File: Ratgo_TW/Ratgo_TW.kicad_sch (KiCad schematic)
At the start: 11 parts, among them J1 10118193-0001LF, J2 Screw_Terminal_01x03, J3 Conn_01x04, Q1 2N7002, Q2 AO3400A, SW1 SW_Push, SW2 SW_Push, U3 AP2112K-3.3, U4 ESP-12F

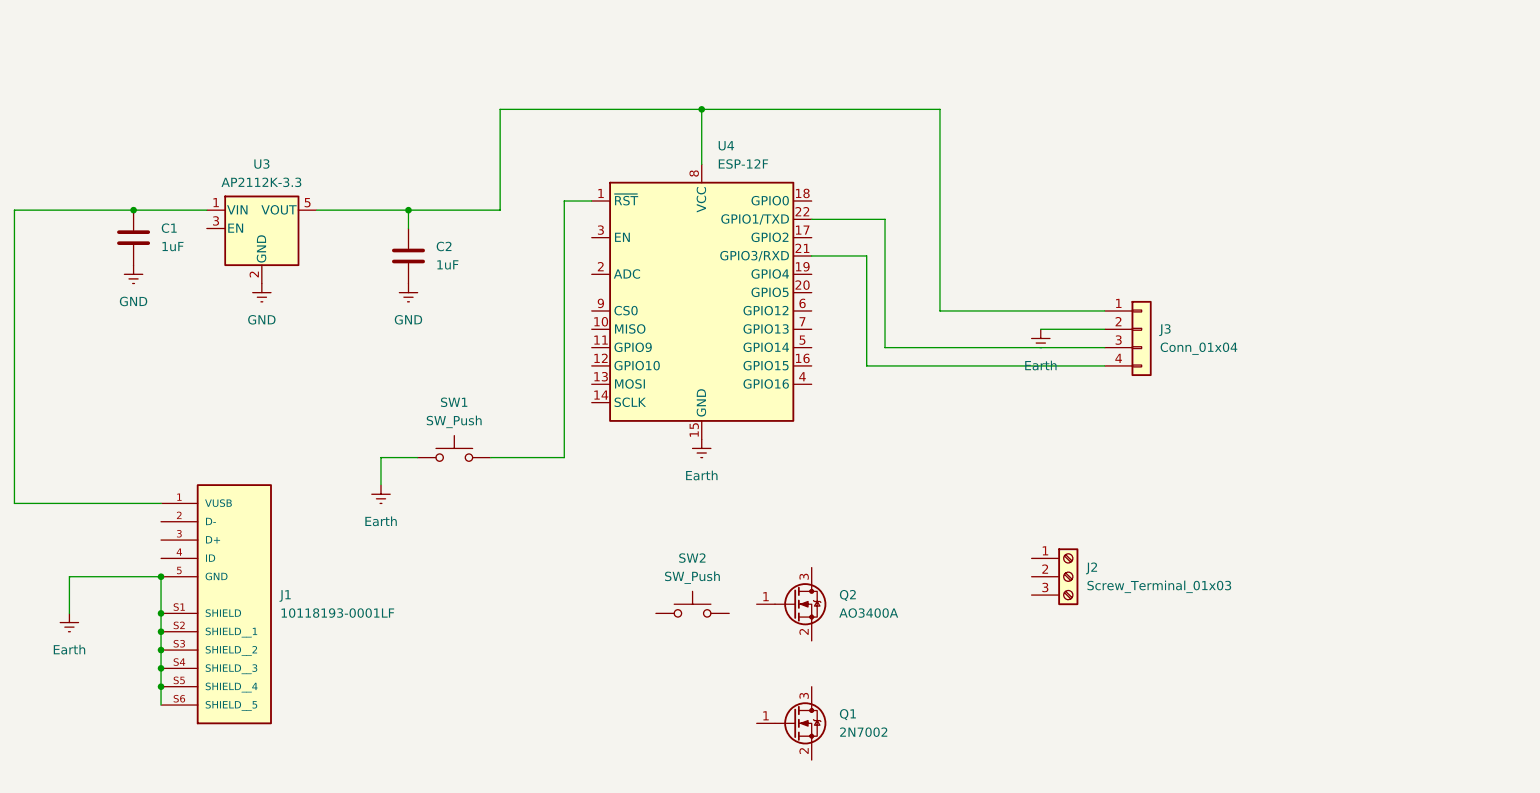
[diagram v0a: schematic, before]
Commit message: latest with all footprints
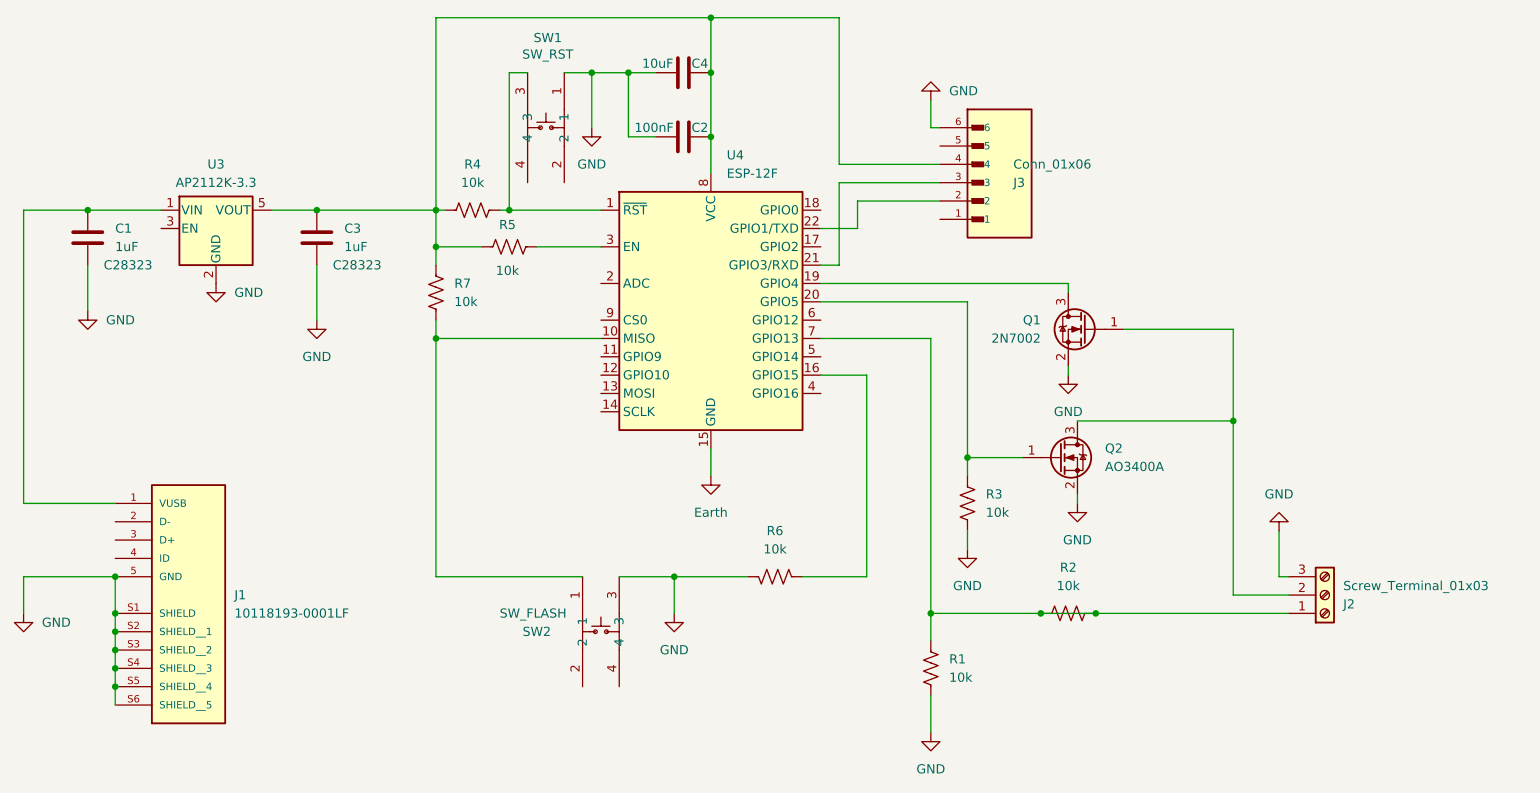
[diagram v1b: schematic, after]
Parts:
- added C3: 1uF, Capacitor_SMD:C_0805_2012Metric, symbol Device:C
- added C4: 10uF, Capacitor_SMD:C_0805_2012Metric, symbol Device:C
- added R1, R2, R3, R4, R5, R6, R7: 10k, Resistor_SMD:R_0805_2012Metric, symbol Device:R_US
- C1: JLCPCB P/N (none) -> C28323
- C2: value 1uF -> 100nF
- J1: footprint 10118193-0001LF:AMPHENOL_10118193-0001LF -> Ratgo2:AMPHENOL_10118193-0001LF
- J2: footprint (none) -> Ratgo2:TB006-508-03BE
- J3: value Conn_01x04 -> Conn_01x06; footprint (none) -> Ratgo2:METZ-CONNECT_PR20206VBNN; symbol Connector_Generic:Conn_01x04 -> Ratgo2:PR20206VBNN; CREATOR (none) -> AAMIR; MANUFACTURER (none) -> Metz Connect; MAXIMUM_PACKAGE_HEIGHT (none) -> 8.6 mm; PARTREV (none) -> Y; STANDARD (none) -> Manufacturer Recommendations; VERIFIER (none) -> RODRIGO
- SW1: value SW_Push -> SW_RST; footprint (none) -> EasyEDA:SW-SMD_4P-L6.2-W6.2-P4.00-LS6.8; symbol Switch:SW_Push -> EasyEDA:SKRAAKE010; LCSC Part (none) -> C115354
- SW2: value SW_Push -> SW_FLASH; footprint (none) -> EasyEDA:SW-SMD_4P-L6.2-W6.2-P4.00-LS6.8; symbol Switch:SW_Push -> EasyEDA:SKRAAKE010; LCSC Part (none) -> C115354
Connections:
- net Earth: no longer J1.5 (GND), J1.S1 (SHIELD), J1.S2 (SHIELD__1), J1.S3 (SHIELD__2), J1.S4 (SHIELD__3), J1.S5 (SHIELD__4), J1.S6 (SHIELD__5), J3.2 (Pin_2), SW1.1
- net GND: now also C2.1, J1.5 (GND), J1.S1 (SHIELD), J1.S2 (SHIELD__1), J1.S3 (SHIELD__2), J1.S4 (SHIELD__3), J1.S5 (SHIELD__4), J1.S6 (SHIELD__5), J2.3 (Pin_3), J3.6, Q1.2 (S), Q2.2 (S), SW1.1, SW2.3, C3.2, C4.1, R1.1, R3.1, R6.1; no longer C2.2
- net at U3.5 (VOUT), U4.8 (VCC): now also C2.2, J3.4, C3.1, C4.2, R4.1, R5.1, R7.1; no longer C2.1, J3.1 (Pin_1)
- net at U4.22 (GPIO1/TXD): now also J3.2; no longer J3.3 (Pin_3)
- net at U4.21 (GPIO3/RXD): now also J3.3; no longer J3.4 (Pin_4)
- net at SW2.1: now also U4.10 (MISO), R7.2
- net at U4.1 (~{RST}): now also SW1.3, R4.2; no longer SW1.2
- net at U4.16 (GPIO15): now also R6.2
- net at U4.19 (GPIO4): now also Q1.3 (D)
- net at U4.20 (GPIO5): now also Q2.1 (G), R3.2
- net at U4.3 (EN): now also R5.2
- net at U4.7 (GPIO13): now also J2.1 (Pin_1), R1.2, R2.1, R2.2
- net at Q1.1 (G): now also J2.2 (Pin_2), Q2.3 (D)
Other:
- moved on the sheet: C1, J1, J2, Q1, Q2, U3, U4
